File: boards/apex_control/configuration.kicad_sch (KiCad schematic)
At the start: 0 parts

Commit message: Logan done fo now
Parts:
- added J1: UJ20-C-H-G-SMT-5-P16, APEX_FOOTPRINTS:UJ20-C-H-G-SMT-5-P16_SameSky, symbol APEX_Symbols:UJ20-C-H-G-SMT-5-P16
- added U10: MKL26Z128VFM4, APEX_FOOTPRINTS:MKL26Z128VFM4_QFN32_NXP, symbol APEX_Symbols:MKL26Z128VFM4
- added U11: W25Q64JW, APEX_FOOTPRINTS:W25Q64JW_USON8_Winbond, symbol APEX_Symbols:W25Q64JW
- added U6: MIMXRT1171DVMAB, APEX_FOOTPRINTS:MIMXRT1171DVMAB_BGA, symbol APEX_Symbols:MIMXRT1171DVMAB
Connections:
- new net: U10.25 (PTC4), U6.P5 (GPIO_LPSR_09)
- new net: U10.32 (PTD7), U6.P6 (GPIO_LPSR_02)
- new net: U10.22 (PTC1), U6.T10 (POR_B)
- new net: U10.26 (PTC5), U6.T6 (GPIO_LPSR_14)
- new net: U10.1 (PTE0), U6.T7 (GPIO_LPSR_03)
- new net: U10.27 (PTC6), U6.U7 (GPIO_LPSR_15)
- new net: U10.24 (PTC3), U6.U8 (GPIO_LPSR_08)
- new net: U10.16 (VSS), U10.2 (VSS)
- new net: J1.A7 (D-), J1.B7 (D-), U10.3 (USB0_DP)
- new net: J1.A6 (D+), J1.B6 (D+), U10.4 (USB0_DM)

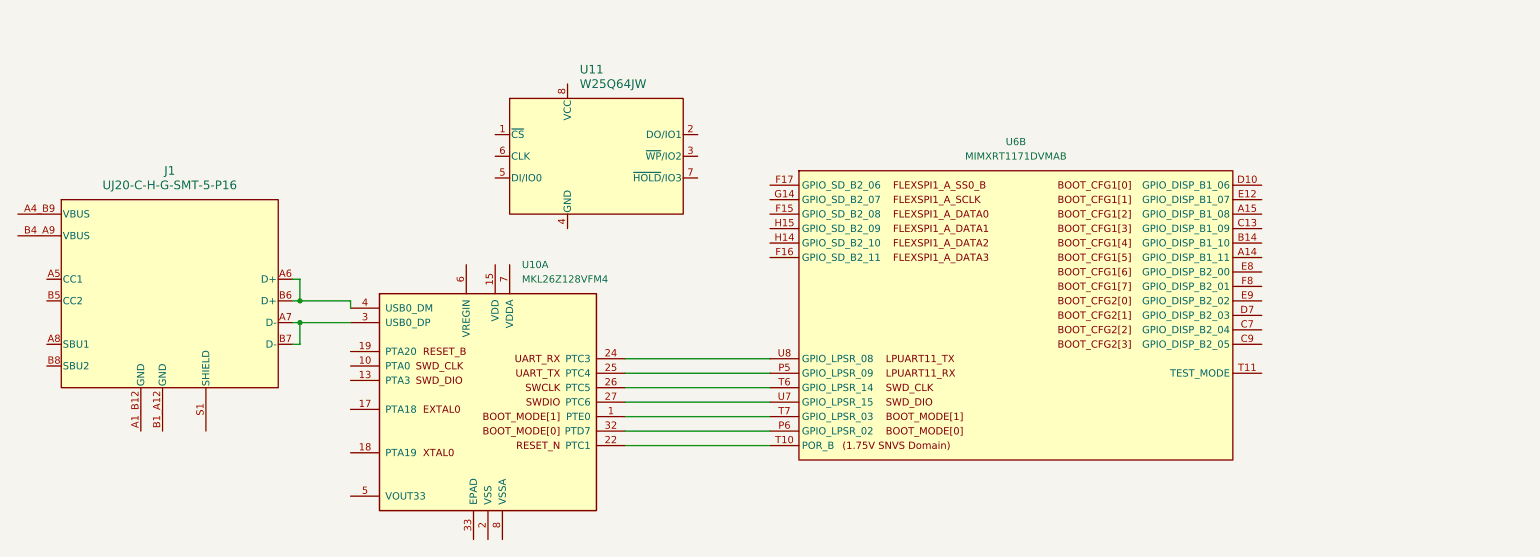
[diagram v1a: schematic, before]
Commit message: More placement
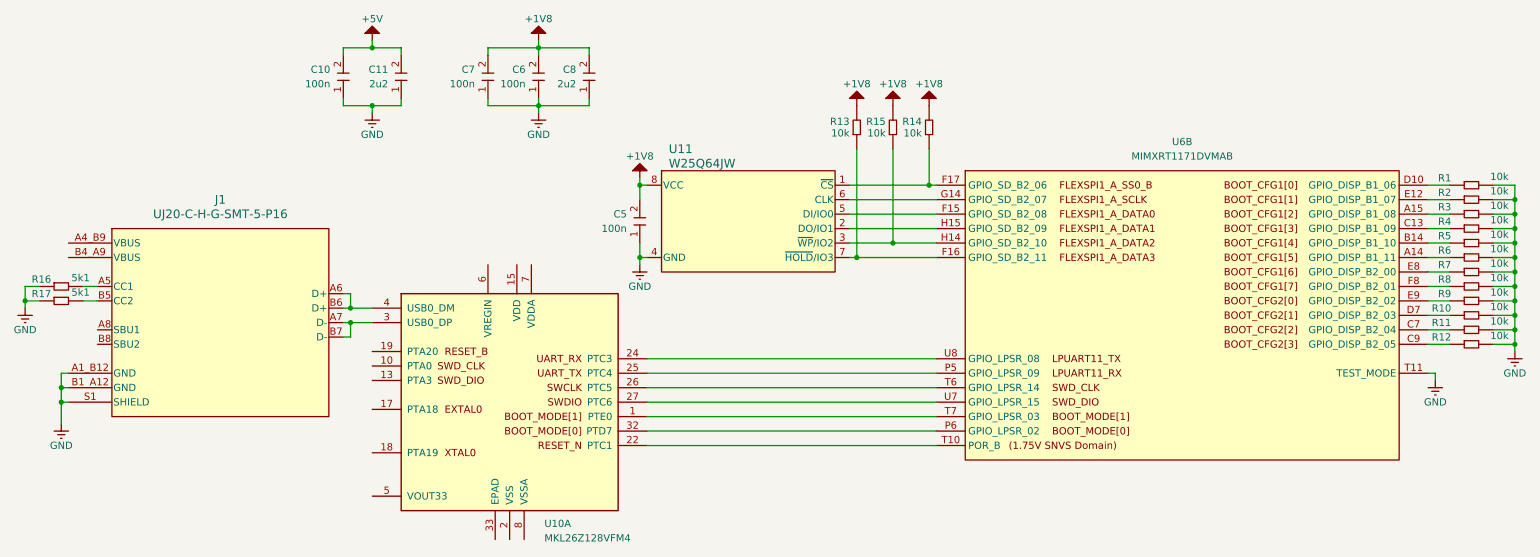
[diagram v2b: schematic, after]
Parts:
- added C10, C5, C6, C7: 100n, symbol APEX_Symbols:C
- added C11, C8: 2u2, symbol APEX_Symbols:C
- added R1, R10, R11, R12, R13, R14, R15, R2, R3, R4, R5, R6, R7, R8, R9: 10k, symbol APEX_Symbols:R
- added R16, R17: 5k1, symbol APEX_Symbols:R
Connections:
- net at U6.A14 (GPIO_DISP_B1_11): now also R6.1
- net at U6.A15 (GPIO_DISP_B1_08): now also R3.1
- net at U6.B14 (GPIO_DISP_B1_10): now also R5.1
- net at U6.C13 (GPIO_DISP_B1_09): now also R4.1
- net at U6.C7 (GPIO_DISP_B2_04): now also R11.1
- net at U6.C9 (GPIO_DISP_B2_05): now also R12.1
- net at U6.D10 (GPIO_DISP_B1_06): now also R1.1
- net at U6.D7 (GPIO_DISP_B2_03): now also R10.1
- net at U6.E12 (GPIO_DISP_B1_07): now also R2.1
- net at U6.E8 (GPIO_DISP_B2_00): now also R7.1
- net at U6.E9 (GPIO_DISP_B2_02): now also R9.1
- net at U6.F15 (GPIO_SD_B2_08): now also U11.5 (DI/IO0)
- net at U6.F16 (GPIO_SD_B2_11): now also U11.7 (~{HOLD}/IO3), R13.1
- net at U6.F17 (GPIO_SD_B2_06): now also U11.1 (~{CS}), R14.1
- net at U6.F8 (GPIO_DISP_B2_01): now also R8.1
- net at U6.G14 (GPIO_SD_B2_07): now also U11.6 (CLK)
- net at U6.H14 (GPIO_SD_B2_10): now also U11.3 (~{WP}/IO2), R15.1
- net at U6.H15 (GPIO_SD_B2_09): now also U11.2 (DO/IO1)
- net GND: now reaches U6.T11 (TEST_MODE)
- net GND: now also J1.A1_B12 (GND), J1.B1_A12 (GND), J1.S1 (SHIELD), U11.4 (GND), C10.1, C11.1, C5.1, C6.1, C7.1, C8.1, R1.2, R10.2, R11.2, R12.2, R16.1, R17.1, R2.2, R3.2, R4.2, R5.2, R6.2, R7.2, R8.2, R9.2
- net +1V8: now reaches U11.8 (VCC)
- net +1V8: now also C5.2, C6.2, C7.2, C8.2, R13.2, R14.2, R15.2
- net at J1.A5 (CC1): now also R16.2
- net at J1.B5 (CC2): now also R17.2
- new net +5V: C10.2, C11.2
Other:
- moved on the sheet: J1, U10A, U11, U6B
